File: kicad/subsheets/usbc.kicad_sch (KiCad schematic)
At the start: 13 parts

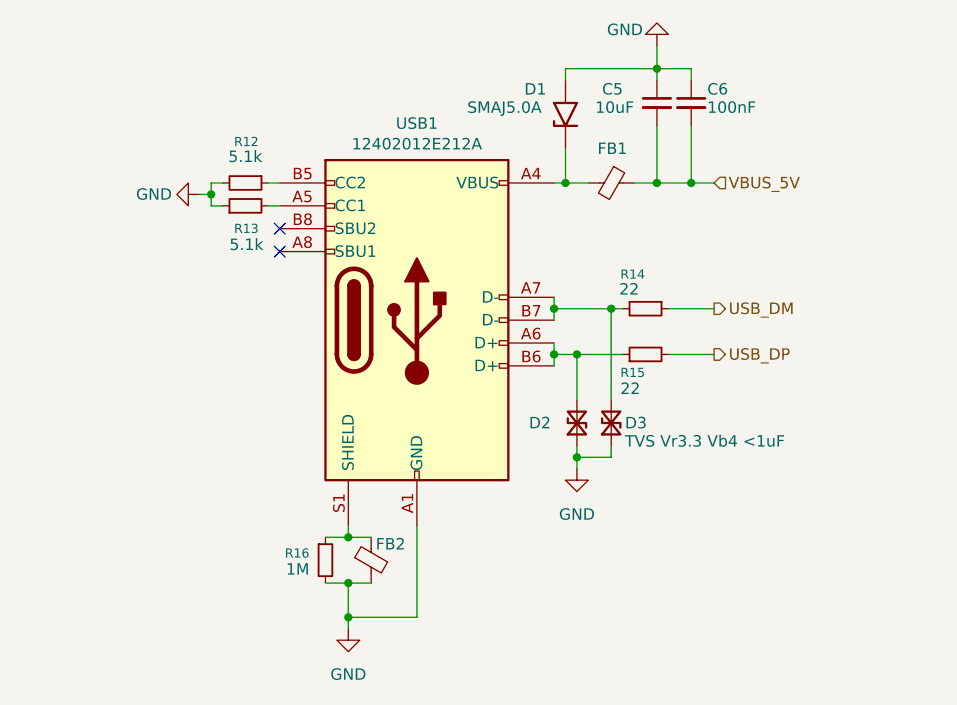
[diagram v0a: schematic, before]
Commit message: Annotations + minor tweaks
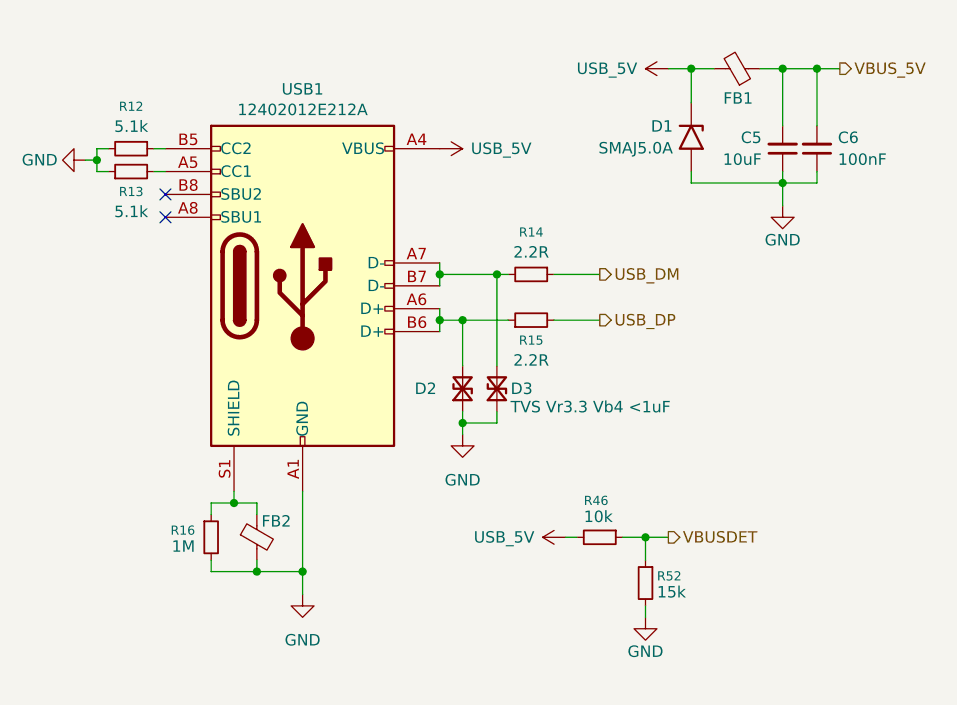
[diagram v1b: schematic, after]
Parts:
- added R46: 10k, symbol Device:R_Small
- added R52: 15k, symbol Device:R_Small
- R14, R15: value 22 -> 2.2R
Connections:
- net GND: now also R52.2
- net USB_5V: now reaches D1.1 (A1), FB1.2, USB1.A4 (VBUS), USB1.A9 (VBUS), USB1.B4 (VBUS), USB1.B9 (VBUS)
- net USB_5V: now also R46.2
- new net VBUSDET: R46.1, R52.1
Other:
- moved on the sheet: C5, C6, D1, D2, D3, FB1, FB2, R12, R13, R14, R15, R16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
